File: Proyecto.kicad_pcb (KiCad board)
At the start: 2 copper layers, 52 parts, among them P1 CONN_01X03, P2 CONN_01X03, Q1 BC808-40, Q2 BC808-40, U1 MCP2515, U2 MCP2551-I/SN, U3 AMS1117, U4 ACS712, U5 ACS712

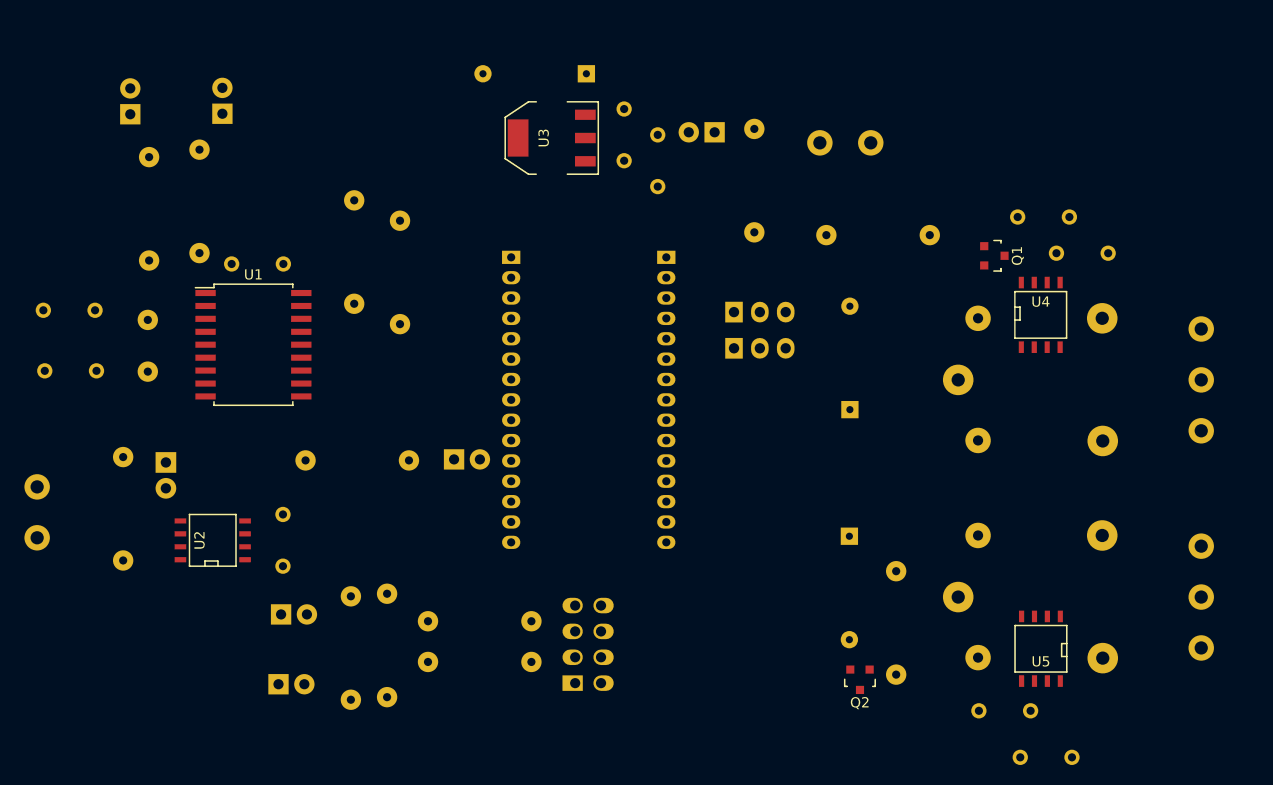
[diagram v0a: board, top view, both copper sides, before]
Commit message: fisx
con 4 puentes... 6.6 cm x12 cm
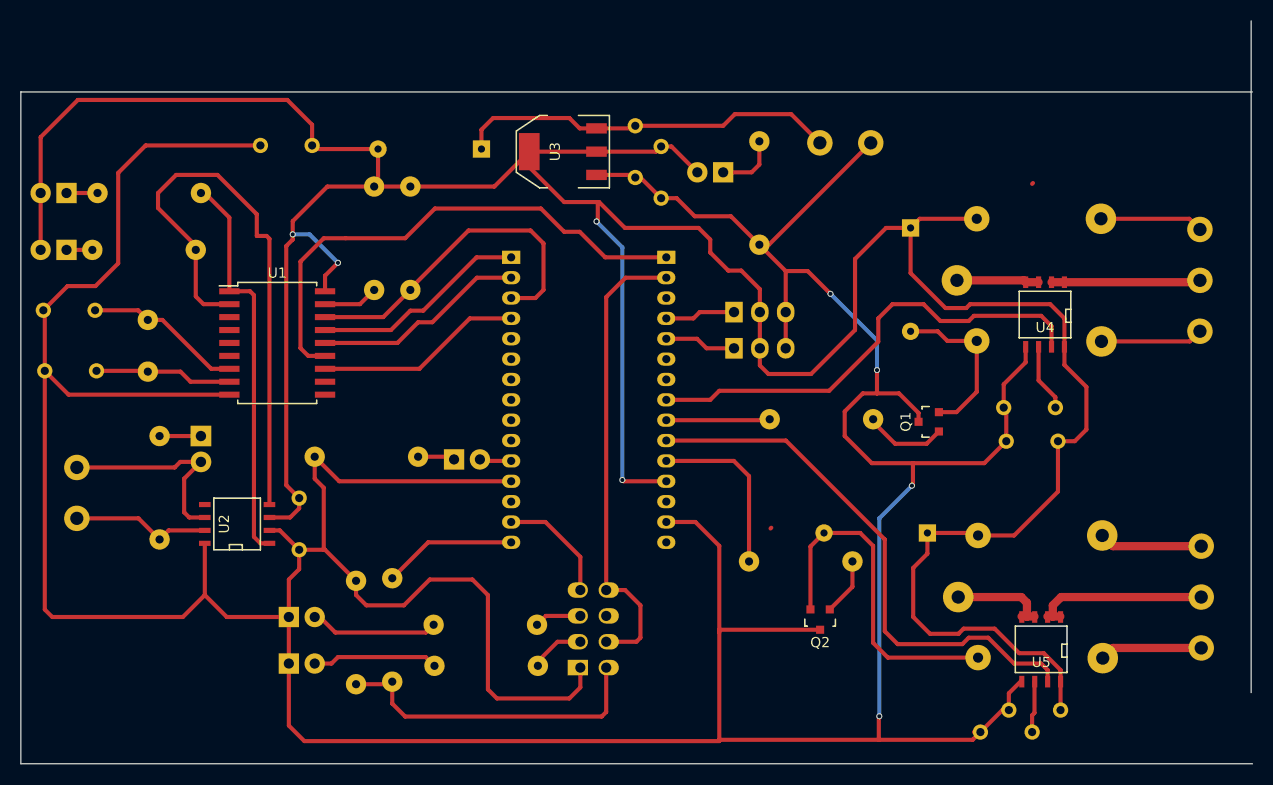
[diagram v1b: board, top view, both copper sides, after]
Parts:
- moved C11 22.1 mm to (157.4, 83.3), turned to 180 degrees
- moved R3 18.9 mm to (136.7, 81.2)
- moved D2 18.8 mm to (145.4, 62.4), turned to 270 degrees
- moved Q1 17.5 mm to (147.2, 81.4), turned to 90 degrees
- moved D_TX1 17.2 mm to (62.5, 58.9), turned to 180 degrees
- moved CFilter1 16.0 mm to (157.1, 80.0), turned to 180 degrees
- moved D_RX1 14.7 mm to (62.5, 64.5), turned to 180 degrees
- moved D1 12.7 mm to (103.3, 54.6)
- moved C7 12.0 mm to (84.1, 54.3)
- moved R4 11.2 mm to (134.6, 95.1), turned to 180 degrees
- moved P1 9.78 mm to (173.8, 67.5)
- moved Relay1 9.78 mm to (150.0, 67.5)
- moved D3 7.67 mm to (147.1, 92.3), turned to 180 degrees
- moved Q2 7.09 mm to (136.5, 100.8)
- moved R8 5.01 mm to (70.6, 58.9), turned to 0 degrees
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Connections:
- Relay1 pad 2: Net-(D2-Pad2) -> +5V
- Relay1 pad 5: +5V -> Net-(D2-Pad2)
- U4 pad 1: Net-(Relay1-Pad1) -> Net-(P1-Pad2)
- U4 pad 2: Net-(Relay1-Pad1) -> Net-(P1-Pad2)
- U4 pad 3: Net-(P1-Pad2) -> Net-(Relay1-Pad1)
- U4 pad 4: Net-(P1-Pad2) -> Net-(Relay1-Pad1)
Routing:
- net GND: track 0.00 -> 451.7 mm, vias 0 -> 4
- net +5V: track 0.00 -> 326.4 mm, vias 0 -> 4
- net Net-(R9-Pad2): track 0.00 -> 57.0 mm
- net /AC2: track 0.00 -> 53.8 mm
- net /SCK: track 0.00 -> 51.3 mm
- net /AC1: track 0.00 -> 46.4 mm
- net /3.3V: track 0.00 -> 46.2 mm
- net Net-(R8-Pad2): track 0.00 -> 39.1 mm
- net Net-(C6-Pad1): track 0.00 -> 37.8 mm
- net Net-(D3-Pad2): track 0.00 -> 33.9 mm
- net /CS: track 0.00 -> 33.7 mm
- net Net-(ESP8266-Pad2): track 0.00 -> 31.9 mm
- net /SO: track 0.00 -> 21.2 mm
- net /SI: track 0.00 -> 20.9 mm
- net /INT: track 0.00 -> 20.3 mm
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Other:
- board outline added: 121 x 73 mm
